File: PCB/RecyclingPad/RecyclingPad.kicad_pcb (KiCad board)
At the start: 2 copper layers, 80.5 x 80.5 mm, 24 parts

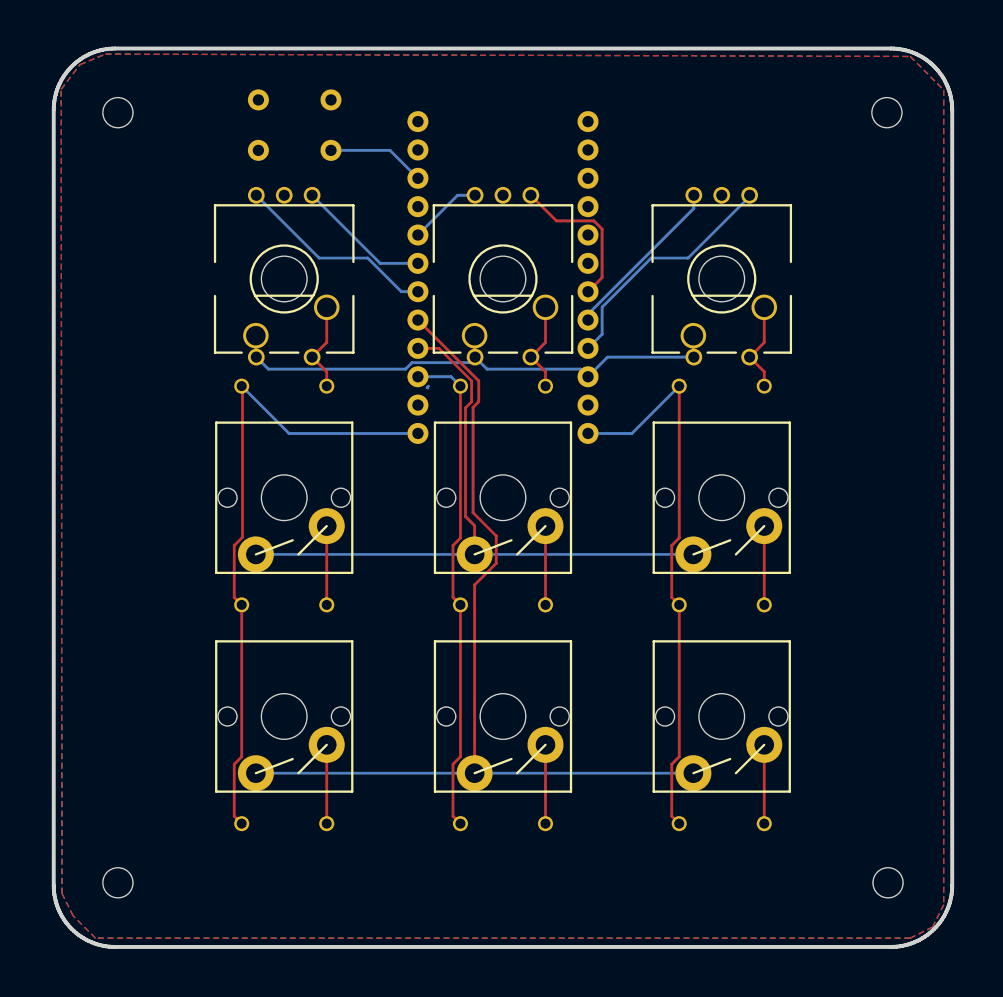
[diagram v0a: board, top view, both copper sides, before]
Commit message: Update recyclingPad v1.0
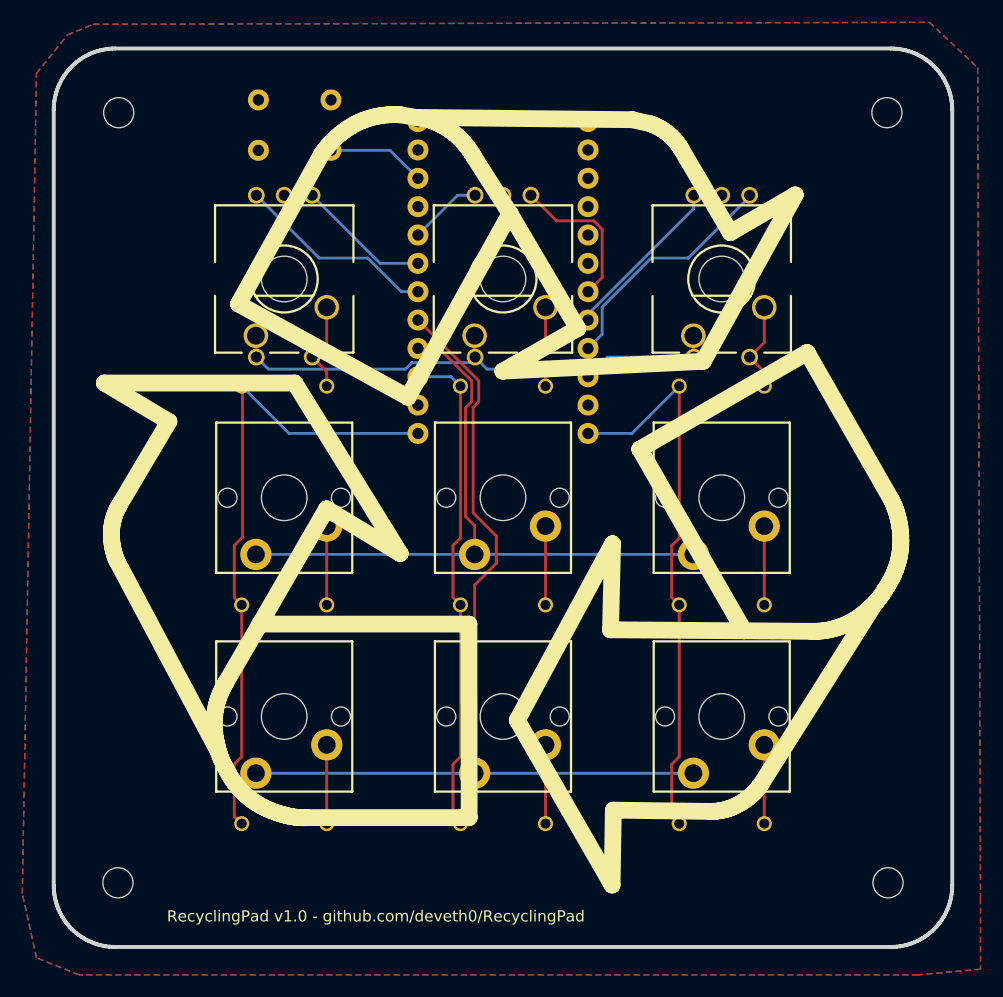
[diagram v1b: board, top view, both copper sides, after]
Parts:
- moved REF** 0.23 mm to (115.6, 65.3)
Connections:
- B1 pad 13: /ROW1 -> /ROW0
- B1 pad 15: /ROW0 -> /ROW1
- D1 pad C: /ROW0 -> /ROW1
- D2 pad C: /ROW0 -> /ROW1
- D3 pad C: /ROW0 -> /ROW1
- D4 pad C: /ROW1 -> /ROW0
- D5 pad C: /ROW1 -> /ROW0
- D6 pad C: /ROW1 -> /ROW0
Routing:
- net /ROW1: track 58.0 -> 44.5 mm
- net /ROW0: track 44.5 -> 58.0 mm
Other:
- board text added: "RecyclingPad v1.0 - github.com/deveth0/RecyclingPad"
- board text removed: "RecyclingPad v0.1 - deveth0"
